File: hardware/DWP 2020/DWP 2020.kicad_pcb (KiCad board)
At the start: 2 copper layers, 97.8 x 77.5 mm, 26 parts, among them K3 SNR03005, K4 SNR03005, T1 TIP32, T2 2SC1815

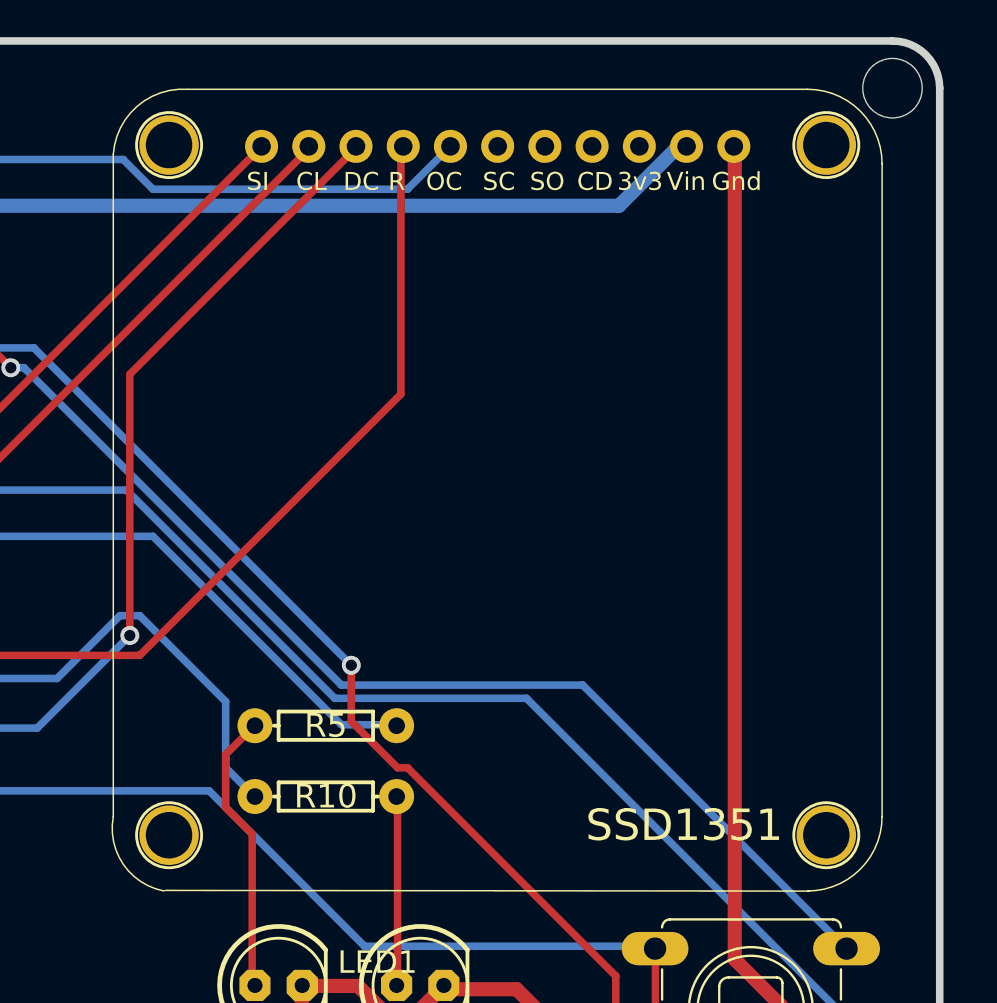
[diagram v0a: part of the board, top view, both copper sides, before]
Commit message: fix some typoos
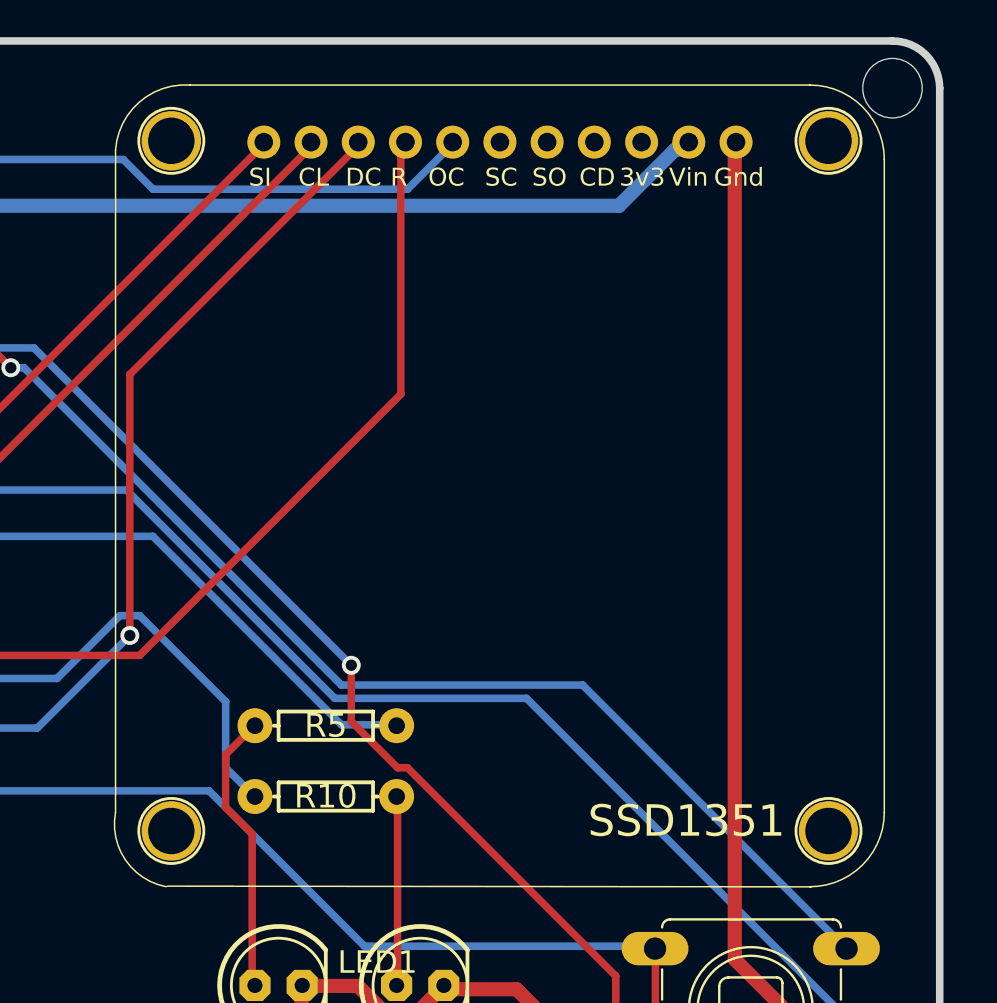
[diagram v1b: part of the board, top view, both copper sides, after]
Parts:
- SSD1351: value SSD1351_128X128_LCD -> SSD1351_128X128; footprint SSD1351_128X128_LCD -> DWP2020 prototype:SSD1351_128X128_LCD
- moved SSD1351 0.26 mm to (172.1, 88.9)
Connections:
- SSD1351 pad JP1$1: D14 -> Net-(SSD1351-PadJP1$1)
- SSD1351 pad JP1$10: D10 -> /D10
- SSD1351 pad JP1$11: D12 -> Net-(SSD1351-PadJP1$11)
- SSD1351 pad JP1$2: D9 -> Net-(SSD1351-PadJP1$2)
- SSD1351 pad JP1$3: (no net) -> Net-(SSD1351-PadJP1$3)
- SSD1351 pad JP1$4: (no net) -> Net-(SSD1351-PadJP1$4)
- SSD1351 pad JP1$5: (no net) -> Net-(SSD1351-PadJP1$5)
- SSD1351 pad JP1$7: VCC -> /VCC
- SSD1351 pad JP1$9: D11 -> Net-(SSD1351-PadJP1$9)
